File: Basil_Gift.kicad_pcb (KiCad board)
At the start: 2 copper layers, 54 x 46 mm, 42 parts, among them J2 693072010801, J3 UJC-H-G1-SMT-P6-TR-67, SW1 Activate, U2 STM32L051C8Tx, U4 TAS2563RPPT, U5 AMS1117, U6 AMS1117

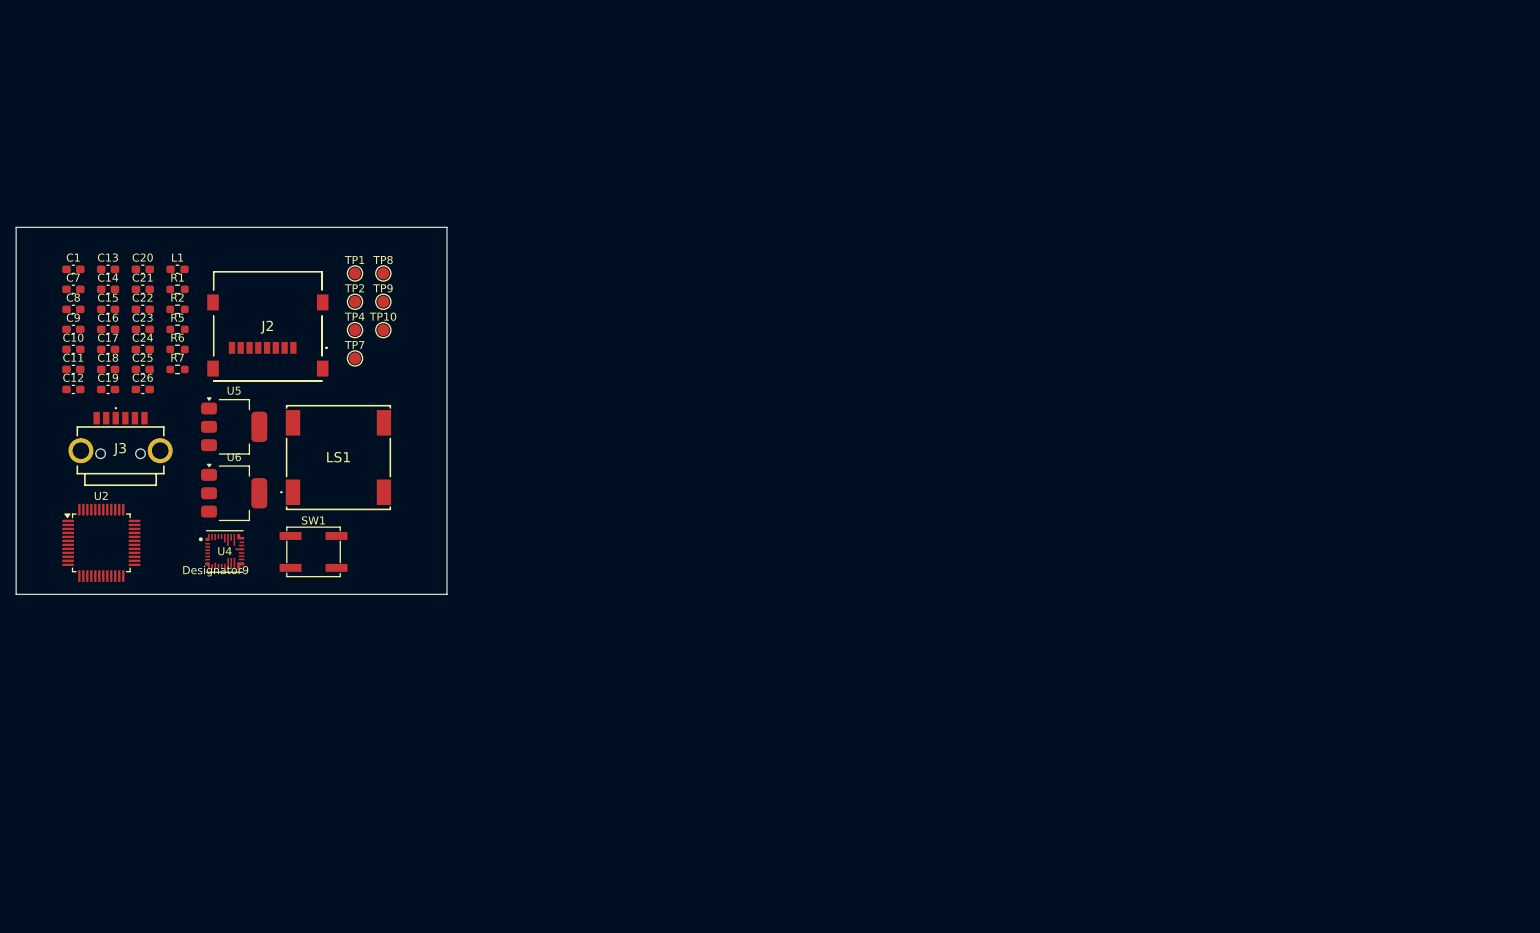
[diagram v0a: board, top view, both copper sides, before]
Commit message: started routing ig
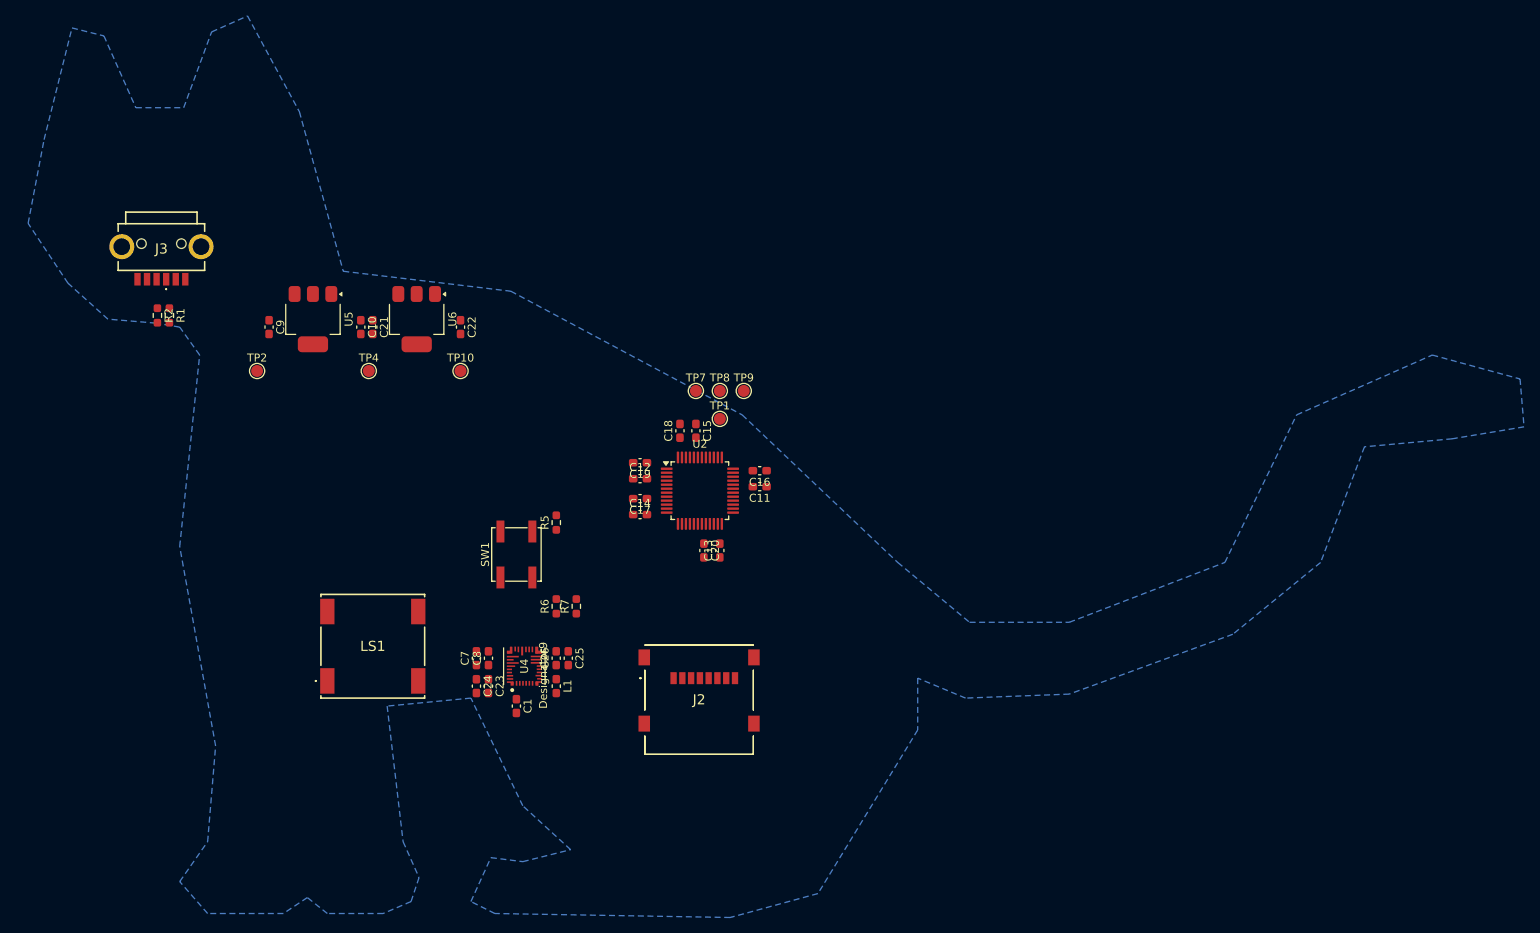
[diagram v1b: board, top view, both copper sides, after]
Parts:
- moved C11 87.3 mm to (150.7, 84.0), turned to 180 degrees
- moved C13 84.4 mm to (145.7, 92.0), turned to 90 degrees
- moved C16 83.6 mm to (150.7, 82.0), turned to 180 degrees
- moved C20 78.7 mm to (143.7, 92.0), turned to -90 degrees
- moved C1 78.0 mm to (120.2, 111.5), turned to -90 degrees
- moved U2 75.3 mm to (143.2, 84.5)
- moved C15 75.2 mm to (142.7, 77.0), turned to -90 degrees
- moved C14 72.4 mm to (135.7, 87.5)
- moved C18 72.1 mm to (140.7, 77.0), turned to 90 degrees
- moved C12 71.9 mm to (135.7, 83.0)
- moved J2 71.5 mm to (143.1, 110.7), turned to 180 degrees
- moved L1 70.6 mm to (125.2, 109.0), turned to -90 degrees
- moved C17 69.2 mm to (135.7, 85.5), turned to 180 degrees
- moved C7 68.5 mm to (115.2, 105.5), turned to 90 degrees
- moved C8 68.0 mm to (116.7, 105.5), turned to 90 degrees
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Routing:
- added copper zone on B.Cu, net GND
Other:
- board outline removed
